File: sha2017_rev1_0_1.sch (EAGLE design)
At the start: 201 parts, among them IC1 CP210X_USB_UART, IC2 LD117AS33TR, IC3 ESP32WROOM32, IC4 TP4056, M1 MOTOR10MM, Q1 MMBT2222A, Q2 MMBT2222A, Q3 MMBT2222A, Q4 MMBT2222A, Q5 SI1304 BDL, Q6 MMBT2222A, T1 MOSFET-PCHANNEL, T2 MOSFET-PCHANNEL, T3 MOSFET-PCHANNEL, U1 MPR121QR2, X2 2908-05WB-MG, X4 JST-PH3

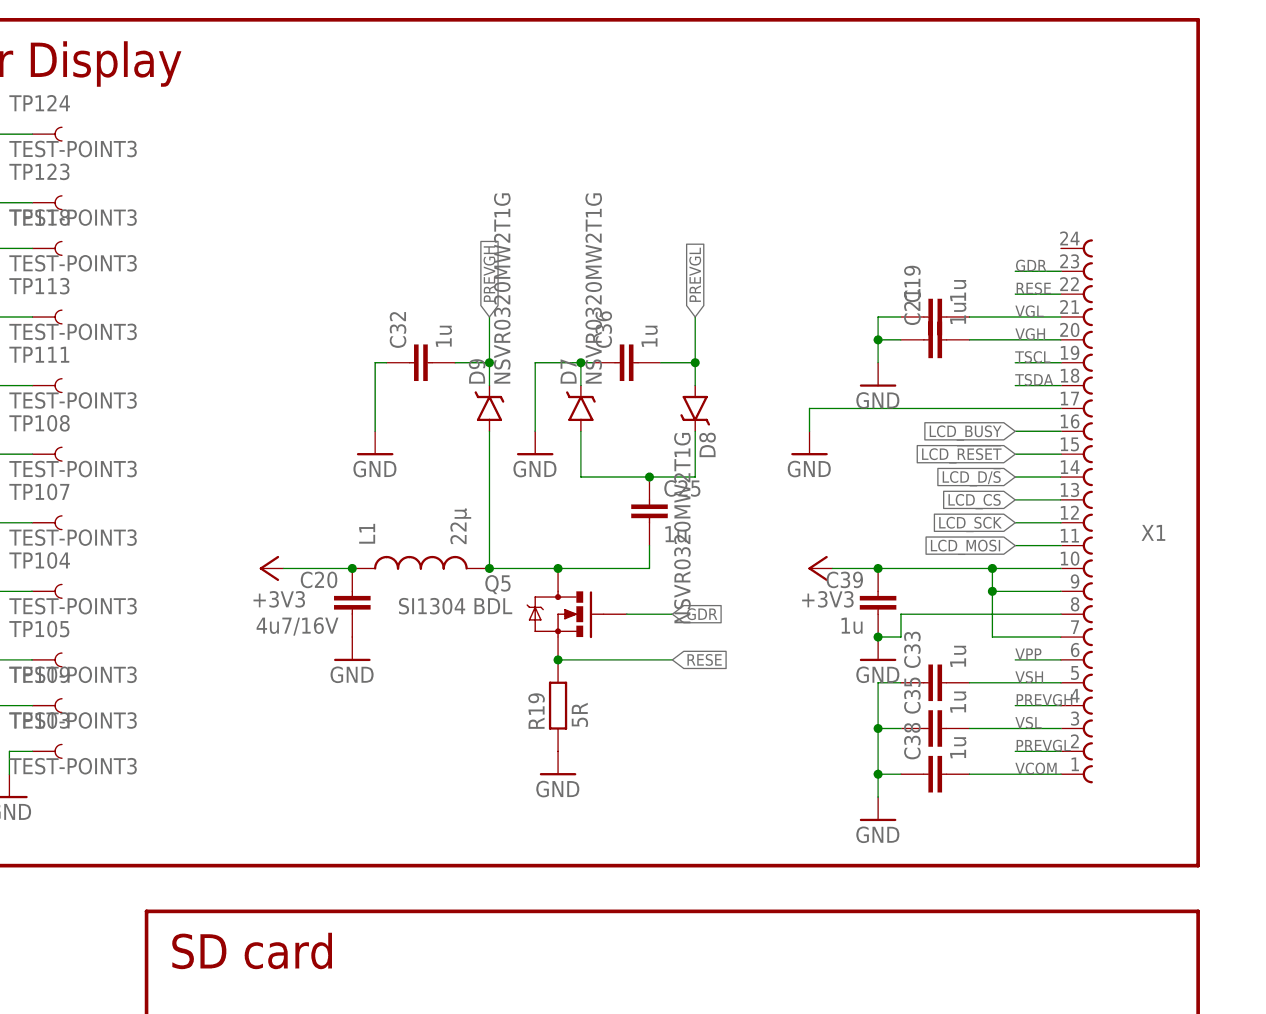
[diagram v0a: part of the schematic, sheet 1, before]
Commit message: Add option for GD/DKE displays - TODO: ROUTE
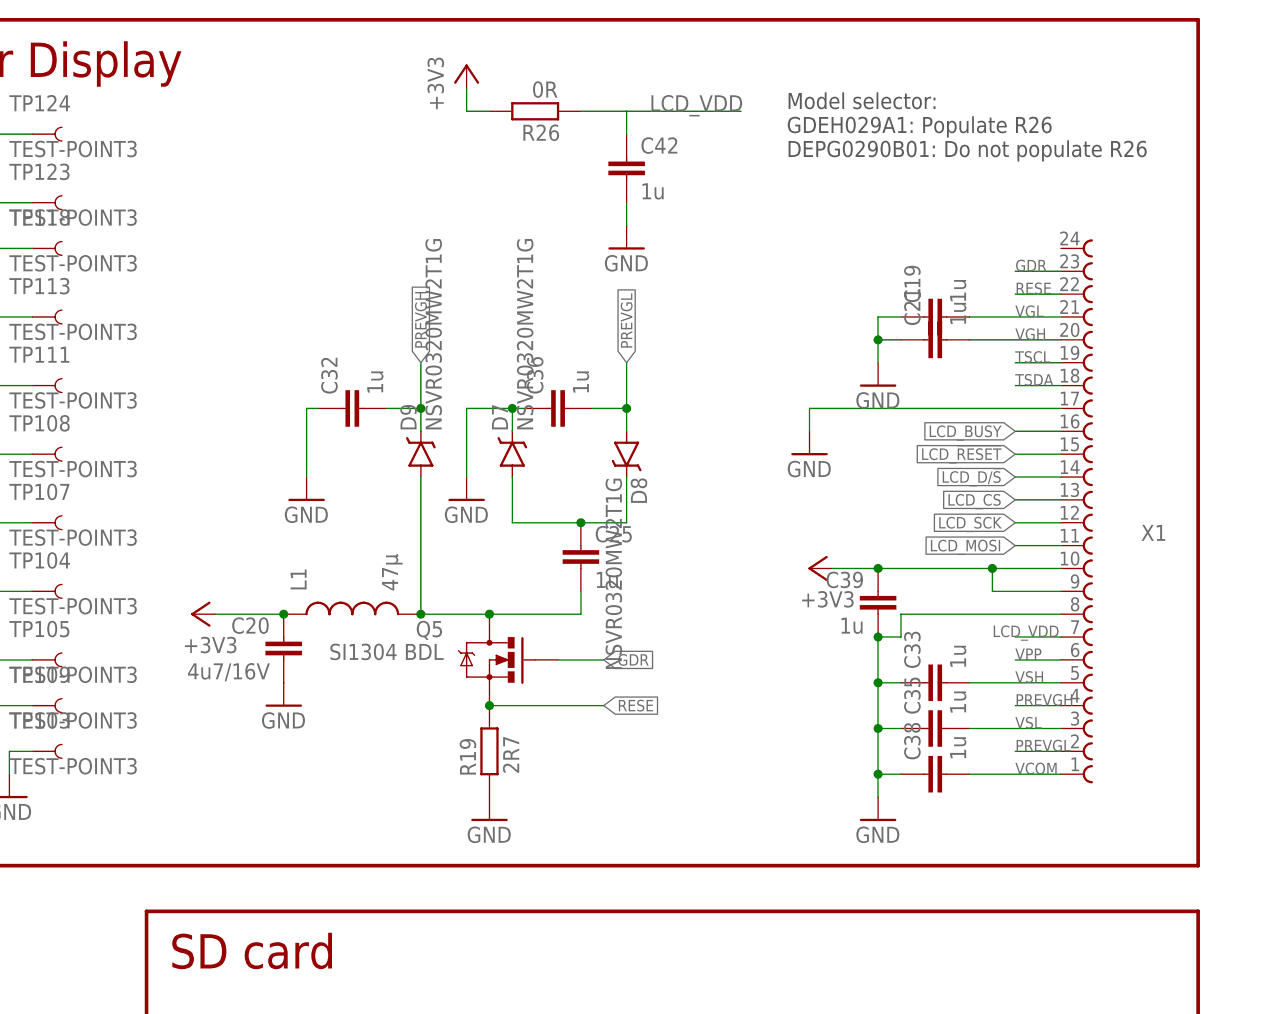
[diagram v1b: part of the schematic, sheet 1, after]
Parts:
- added C42: 1u, sha2017_rev0_1_0_dev:C0603-DASHES
- added R26: 0R, sha2017_rev0_1_0_dev:R0603-DASHES
- L1: value 22µ -> 47µ
- R19: value 5R -> 2R7
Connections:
- new net LCD_VDD: C42.1, R26.2, X1.7
- net +3V3: now also R26.1; no longer X1.7
- net GND: now also C42.2
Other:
- note added: "Model selector: GDEH029A1: Populate R26 DEPG0290B01: Do not populate R26"
- moved on the sheet: C20, C25, C32, C36, D7, D8, D9, L1, Q5, R19
